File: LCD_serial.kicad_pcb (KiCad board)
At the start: 2 copper layers, 5 parts, among them P1 CONN_01X05, U1 74LS164

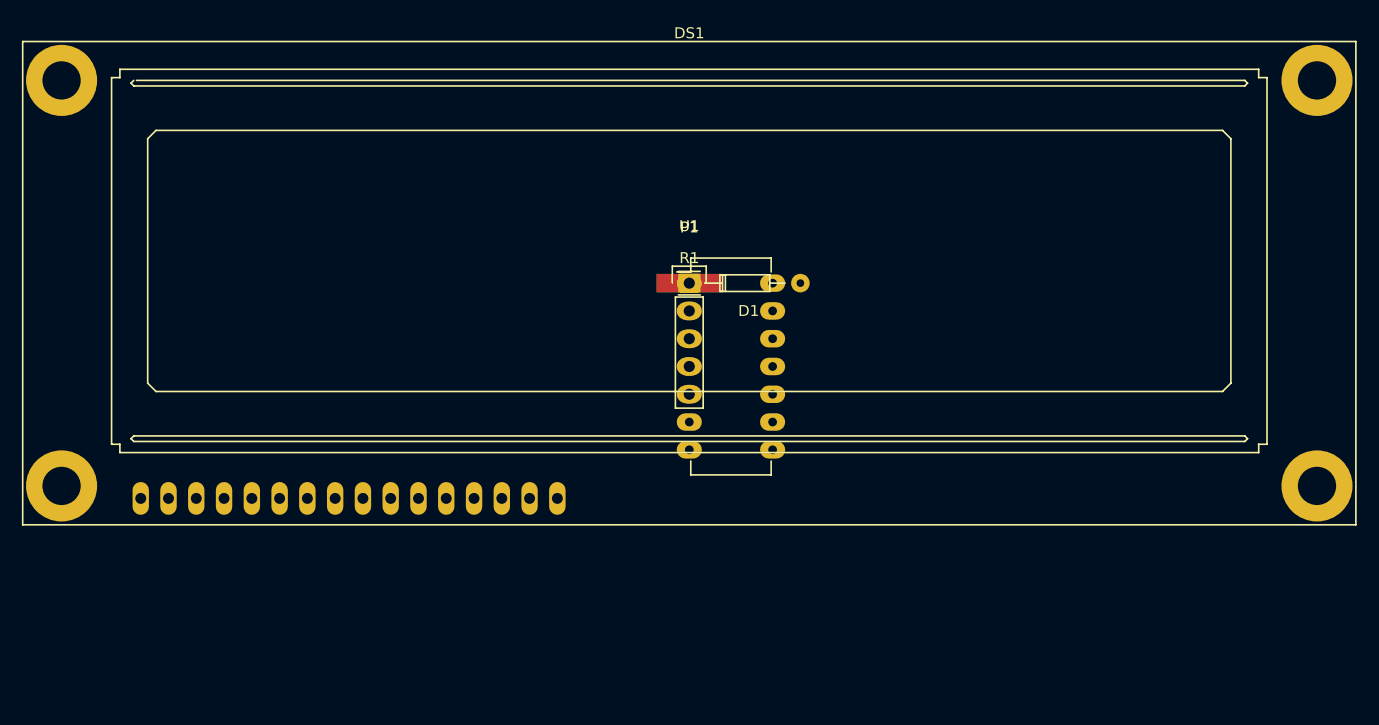
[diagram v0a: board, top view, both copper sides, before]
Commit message: Starting on the PCB layout
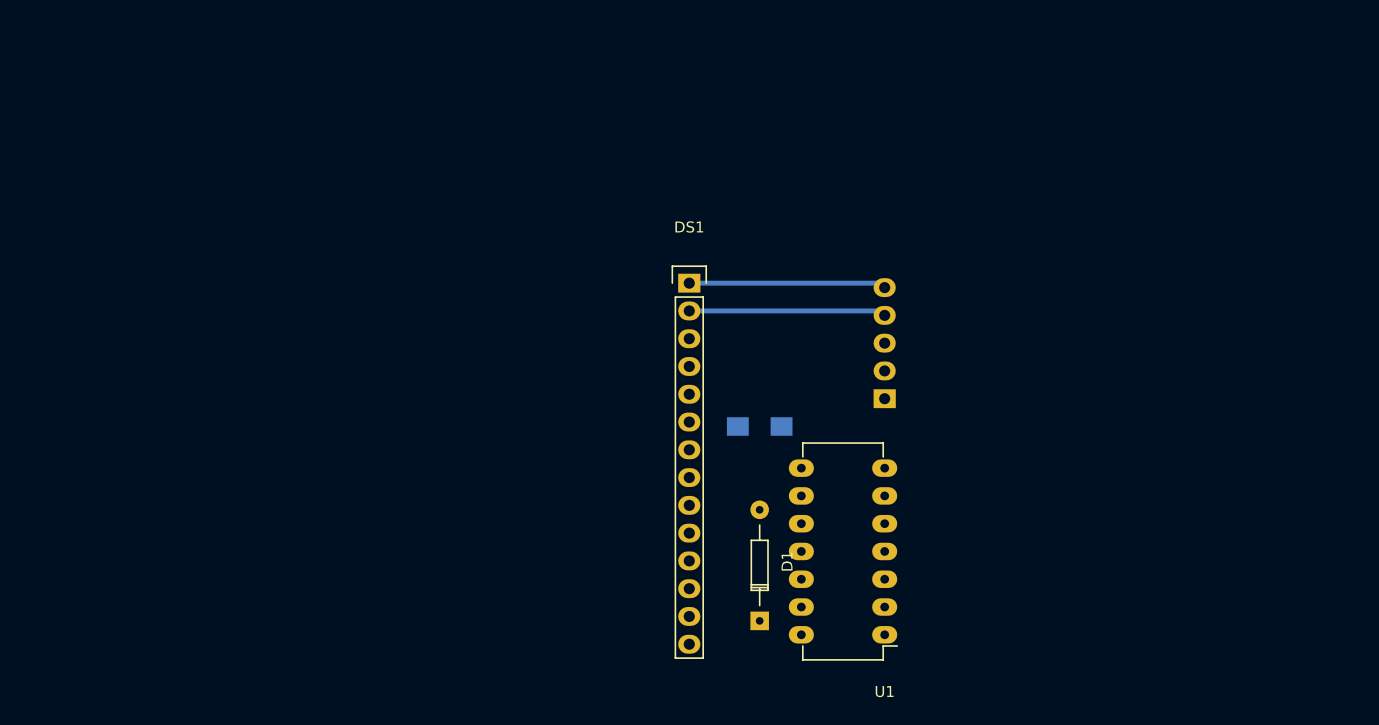
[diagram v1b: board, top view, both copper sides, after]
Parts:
- DS1: footprint Display:LCD-016N002L -> Pin_Headers:Pin_Header_Straight_1x14
- P1, R1: moved to B.Cu
- moved U1 36.8 mm to (166.4, 137.2), turned to 180 degrees
- moved D1 31.6 mm to (154.9, 135.9), turned to 90 degrees
- moved P1 20.8 mm to (166.4, 115.6)
- moved R1 14.6 mm to (154.9, 118.1)
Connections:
- net GND renamed Net-(DS1-Pad1)
- net VCC renamed Net-(DS1-Pad2)
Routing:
- net Net-(DS1-Pad2): track 0.00 -> 18.0 mm
- net Net-(DS1-Pad1): track 0.00 -> 18.0 mm
